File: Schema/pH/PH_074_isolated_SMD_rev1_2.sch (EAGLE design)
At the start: 32 parts, among them IC1 TL074D, IC2 TLC271D

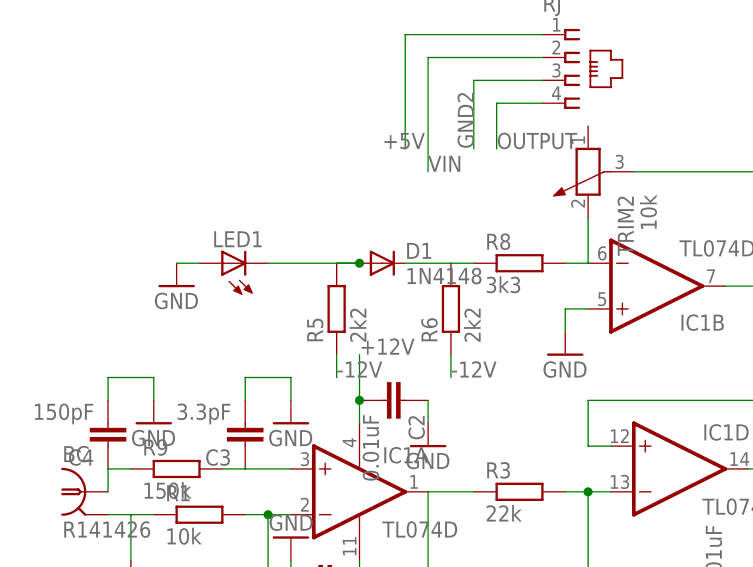
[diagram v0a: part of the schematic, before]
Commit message: add Shield
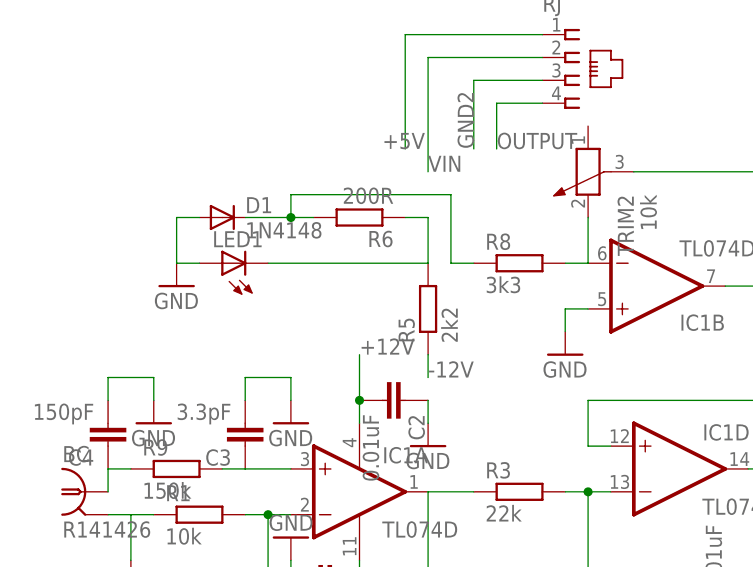
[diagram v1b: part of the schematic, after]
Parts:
- R6: value 2k2 -> 200R
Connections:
- net -12V: no longer R6.1
- net GND: now also D1.A
- net N$8: now also R6.1; no longer D1.A
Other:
- moved on the sheet: D1, R5, R6
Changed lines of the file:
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@@
 <part name="R3" library="rcl" deviceset="R-EU_" device="R1206W" value="22k"/>
 <part name="R5" library="rcl" deviceset="R-EU_" device="R1206W" value="2k2"/>
-<part name="R6" library="rcl" deviceset="R-EU_" device="R1206W" value="2k2"/>
+<part name="R6" library="rcl" deviceset="R-EU_" device="R1206W" value="200R"/>
 <part name="C1" library="rcl" deviceset="C-EU" device="C1206" value="0.01uF"/>
 <part name="R4" library="rcl" deviceset="R-EU_" device="R1206W" value="22k"/>
@@
 <instance part="TRIM2" gate="1" x="48.26" y="63.5" rot="MR270"/>
 <instance part="R3" gate="G$1" x="40.64" y="27.94"/>
-<instance part="R5" gate="G$1" x="20.32" y="48.26" rot="R90"/>
-<instance part="R6" gate="G$1" x="33.02" y="48.26" rot="R90"/>
+<instance part="R5" gate="G$1" x="30.48" y="48.26" rot="R90"/>
+<instance part="R6" gate="G$1" x="22.86" y="58.42" rot="R180"/>
 <instance part="C1" gate="G$1" x="58.42" y="15.24" rot="R90"/>
 <instance part="R4" gate="G$1" x="58.42" y="7.62" rot="R180"/>
@@
 <instance part="GND8" gate="1" x="45.72" y="43.18"/>
 <instance part="R8" gate="G$1" x="40.64" y="53.34"/>
-<instance part="D1" gate="G$1" x="25.4" y="53.34"/>
+<instance part="D1" gate="G$1" x="7.62" y="58.42"/>
 <instance part="LED1" gate="G$1" x="10.16" y="53.34" rot="R90"/>
 <instance part="IL300" gate="A" x="137.16" y="25.4"/>
@@
 <pinref part="LED1" gate="G$1" pin="A"/>
 <wire x1="2.54" y1="53.34" x2="5.08" y2="53.34" width="0.1524" layer="91"/>
+<wire x1="2.54" y1="53.34" x2="2.54" y2="58.42" width="0.1524" layer="91"/>
+<pinref part="D1" gate="G$1" pin="A"/>
+<wire x1="2.54" y1="58.42" x2="5.08" y2="58.42" width="0.1524" layer="91"/>
 </segment>
 </net>
@@
 </segment>
 <segment>
-<wire x1="20.32" y1="40.64" x2="20.32" y2="43.18" width="0.1524" layer="91"/>
-<label x="20.32" y="40.64" size="1.778" layer="95"/>
+<wire x1="30.48" y1="40.64" x2="30.48" y2="43.18" width="0.1524" layer="91"/>
+<label x="30.48" y="40.64" size="1.778" layer="95"/>
 <pinref part="R5" gate="G$1" pin="1"/>
-</segment>
-<segment>
-<wire x1="33.02" y1="40.64" x2="33.02" y2="43.18" width="0.1524" layer="91"/>
-<label x="33.02" y="40.64" size="1.778" layer="95"/>
-<pinref part="R6" gate="G$1" pin="1"/>
 </segment>
 </net>
@@
 </segment>
 </net>
-<net name="N$8" class="0">
-<segment>
-<pinref part="R5" gate="G$1" pin="2"/>
-<pinref part="LED1" gate="G$1" pin="C"/>
-<wire x1="12.7" y1="53.34" x2="22.86" y2="53.34" width="0.1524" layer="91"/>
-<pinref part="D1" gate="G$1" pin="A"/>
-<junction x="22.86" y="53.34"/>
-<wire x1="22.86" y1="53.34" x2="20.32" y2="53.34" width="0.1524" layer="91"/>
-</segment>
-</net>
-<net name="N$7" class="0">
-<segment>
-<pinref part="D1" gate="G$1" pin="C"/>
-<pinref part="R6" gate="G$1" pin="2"/>
-<wire x1="27.94" y1="53.34" x2="33.02" y2="53.34" width="0.1524" layer="91"/>
-<pinref part="R8" gate="G$1" pin="1"/>
-<wire x1="35.56" y1="53.34" x2="33.02" y2="53.34" width="0.1524" layer="91"/>
-</segment>
-</net>
 <net name="N$5" class="0">
 <segment>
@@
 </segment>
 </net>
+<net name="N$8" class="0">
+<segment>
+<pinref part="LED1" gate="G$1" pin="C"/>
+<pinref part="R5" gate="G$1" pin="2"/>
+<wire x1="12.7" y1="53.34" x2="30.48" y2="53.34" width="0.1524" layer="91"/>
+<pinref part="R6" gate="G$1" pin="1"/>
+<wire x1="27.94" y1="58.42" x2="30.48" y2="58.42" width="0.1524" layer="91"/>
+<wire x1="30.48" y1="58.42" x2="30.48" y2="53.34" width="0.1524" layer="91"/>
+</segment>
+</net>
+<net name="N$7" class="0">
+<segment>
+<pinref part="D1" gate="G$1" pin="C"/>
+<pinref part="R6" gate="G$1" pin="2"/>
+<wire x1="10.16" y1="58.42" x2="15.24" y2="58.42" width="0.1524" layer="91"/>
+<pinref part="R8" gate="G$1" pin="1"/>
+<wire x1="15.24" y1="58.42" x2="17.78" y2="58.42" width="0.1524" layer="91"/>
+<wire x1="35.56" y1="53.34" x2="33.02" y2="53.34" width="0.1524" layer="91"/>
+<wire x1="33.02" y1="53.34" x2="33.02" y2="60.96" width="0.1524" layer="91"/>
+<wire x1="33.02" y1="60.96" x2="15.24" y2="60.96" width="0.1524" layer="91"/>
+<wire x1="15.24" y1="60.96" x2="15.24" y2="58.42" width="0.1524" layer="91"/>
+<junction x="15.24" y="58.42"/>
+</segment>
+</net>
